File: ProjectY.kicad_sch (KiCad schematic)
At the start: 10 parts, among them J10 NRJ6HF, J2 Conn_ARM_JTAG_SWD_10, J3 9V, J4 NRJ6HF, J5 NRJ6HF, J6 NRJ6HF, J7 SPDIF_OUT, J8 Midi In, J9 MIDI Out, P1 USB_C

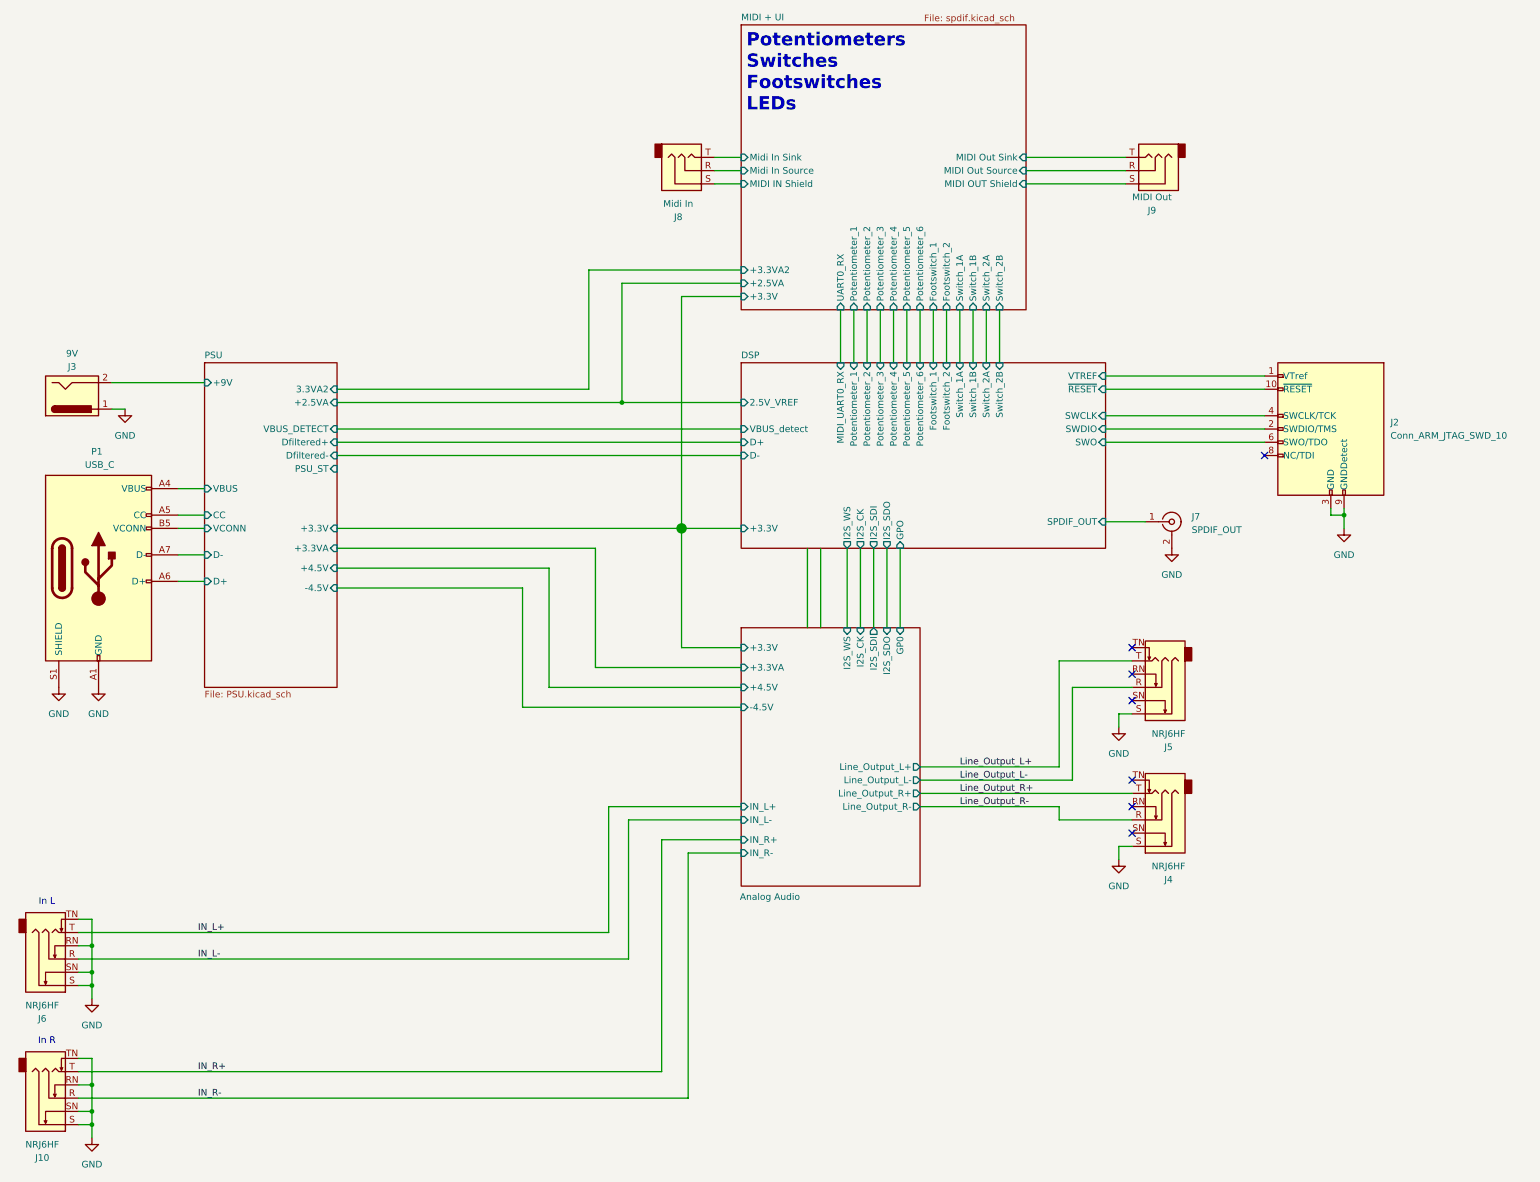
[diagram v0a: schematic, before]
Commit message: started the layout process
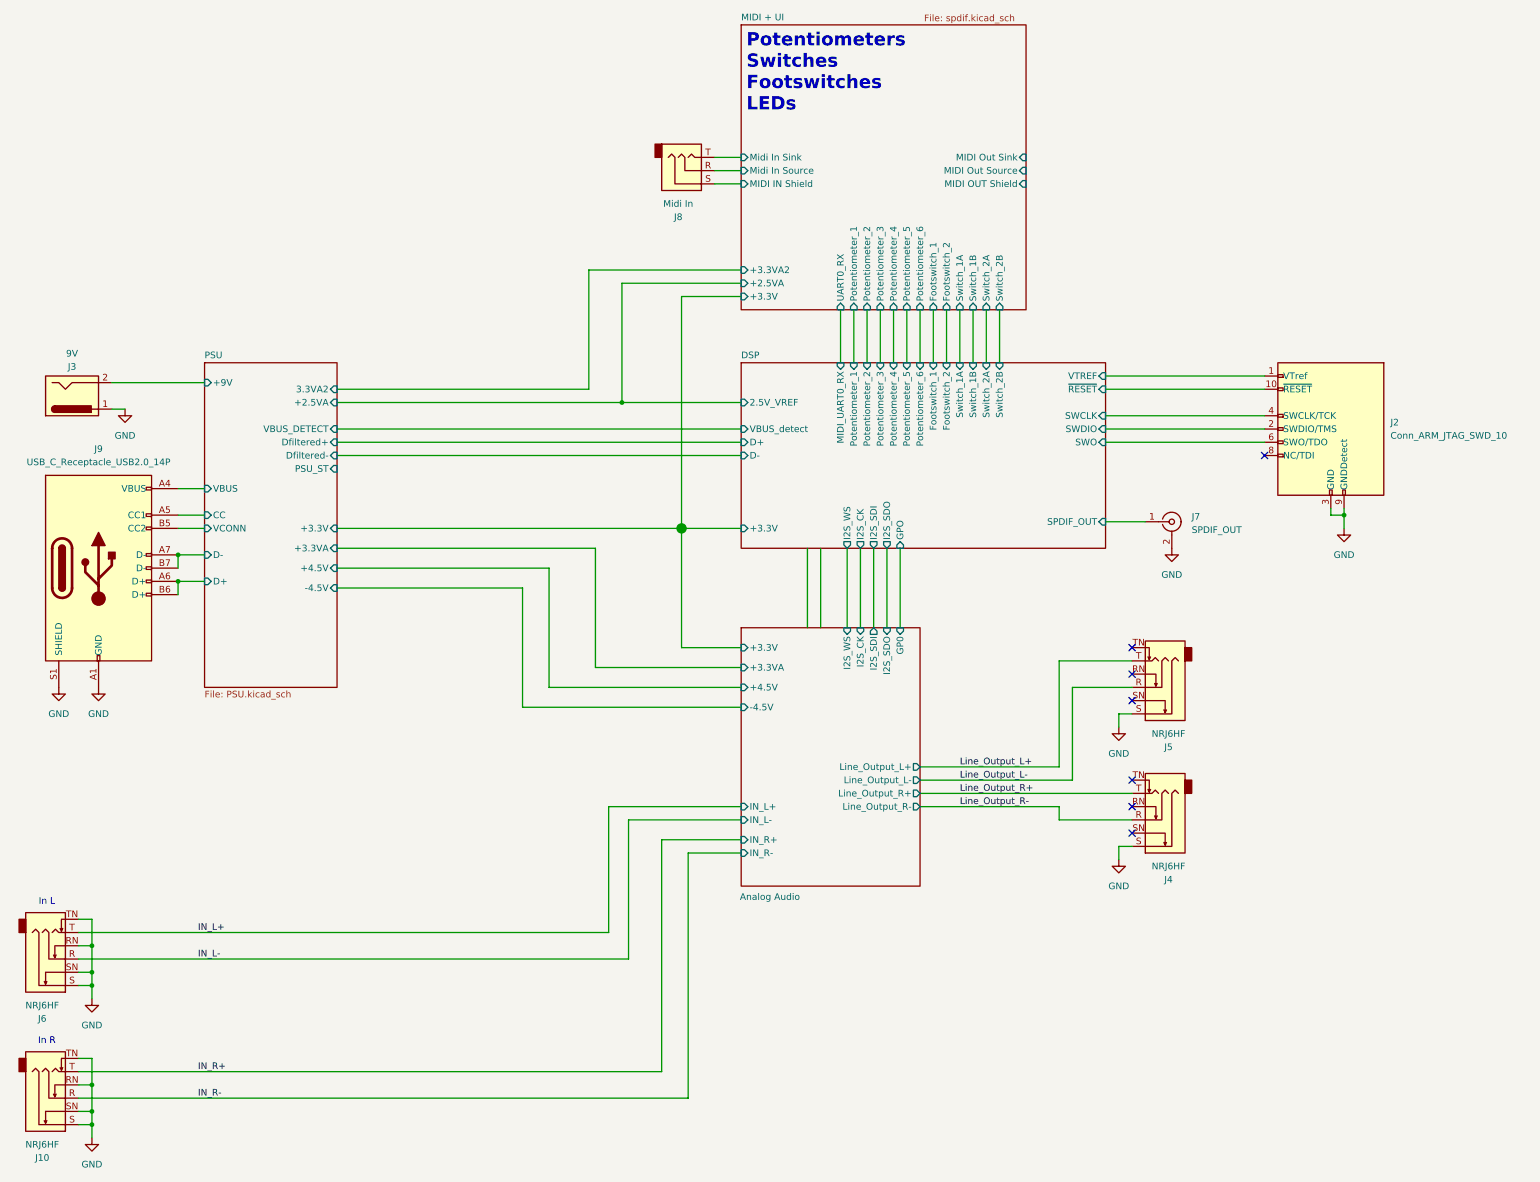
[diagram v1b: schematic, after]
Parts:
- removed J9: MIDI Out, Connector_Audio:Jack_3.5mm_Lumberg_1503_07_Horizontal, symbol Connector_Audio:AudioJack3
- removed P1: USB_C, Connector_USB:USB_C_Receptacle_GCT_USB4110, symbol Connector:USB_C_Plug_USB2.0
- added J9: USB_C_Receptacle_USB2.0_14P, Connector_USB:USB_C_Receptacle_GCT_USB4110, symbol Connector:USB_C_Receptacle_USB2.0_14P
- J2: footprint (none) -> Connector_PinHeader_1.27mm:PinHeader_2x05_P1.27mm_Vertical_SMD
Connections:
- net GND: now also J9.A1 (GND), J9.A12 (GND), J9.B1 (GND), J9.B12 (GND), J9.S1 (SHIELD)
- net PSU/CC: now also J9.A5 (CC1)
- net PSU/D+: now also J9.A6 (D+), J9.B6 (D+)
- net PSU/D-: now also J9.A7 (D-), J9.B7 (D-)
- net PSU/VBUS: now also J9.A4 (VBUS), J9.A9 (VBUS), J9.B4 (VBUS), J9.B9 (VBUS)
- net PSU/VCONN: now also J9.B5 (CC2)
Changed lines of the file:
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@@
+	)
+	(junction
+		(at 100.33 144.78)
+		(diameter 0)
+		(color 0 0 0 0)
 	)
 	(junction
@@
 		(color 255 0 0 1)
 	)
+	(junction
+		(at 100.33 149.86)
+		(diameter 0)
+		(color 0 0 0 0)
+	)
 	(no_connect
 		(at 308.61 125.73)
@@
 	(wire
 		(pts
+			(xy 100.33 147.32) (xy 100.33 144.78)
+		)
+		(stroke
+			(width 0)
+			(type default)
+		)
+	)
+	(wire
+		(pts
 			(xy 283.21 170.18) (xy 271.78 170.18)
 		)
@@
 	(wire
 		(pts
-			(xy 262.89 71.12) (xy 281.94 71.12)
-		)
-		(stroke
-			(width 0)
-			(type default)
-		)
-	)
-	(wire
-		(pts
 			(xy 171.45 147.32) (xy 171.45 170.18)
 		)
@@
 	(wire
 		(pts
+			(xy 100.33 144.78) (xy 105.41 144.78)
+		)
+		(stroke
+			(width 0)
+			(type default)
+		)
+	)
+	(wire
+		(pts
 			(xy 233.68 143.51) (xy 233.68 158.75)
 		)
@@
 	(wire
 		(pts
-			(xy 262.89 73.66) (xy 281.94 73.66)
-		)
-		(stroke
-			(width 0)
-			(type default)
-		)
-	)
-	(wire
-		(pts
 			(xy 182.88 193.04) (xy 208.28 193.04)
 		)
@@
 	(wire
 		(pts
-			(xy 262.89 68.58) (xy 281.94 68.58)
-		)
-		(stroke
-			(width 0)
-			(type default)
-		)
-	)
-	(wire
-		(pts
 			(xy 208.28 95.25) (xy 196.85 95.25)
 		)
@@
 	(wire
 		(pts
-			(xy 100.33 144.78) (xy 105.41 144.78)
-		)
-		(stroke
-			(width 0)
-			(type default)
-		)
-	)
-	(wire
-		(pts
 			(xy 83.82 241.3) (xy 83.82 246.38)
 		)
@@
 		(pts
 			(xy 130.81 147.32) (xy 171.45 147.32)
+		)
+		(stroke
+			(width 0)
+			(type default)
+		)
+	)
+	(wire
+		(pts
+			(xy 100.33 149.86) (xy 100.33 152.4)
 		)
 		(stroke
@@
 	)
 	(symbol
+		(lib_id "Connector:USB_C_Receptacle_USB2.0_14P")
+		(at 85.09 147.32 0)
+		(unit 1)
+		(exclude_from_sim no)
+		(in_bom yes)
+		(on_board yes)
+		(dnp no)
+		(fields_autoplaced yes)
+		(property "Reference" "J9"
+			(at 85.09 124.46 0)
+			(effects
+				(font
+					(size 1.27 1.27)
+				)
+			)
+		)
+		(property "Value" "USB_C_Receptacle_USB2.0_14P"
+			(at 85.09 127 0)
+			(effects
+				(font
+					(size 1.27 1.27)
+				)
+			)
+		)
+		(property "Footprint" "Connector_USB:USB_C_Receptacle_GCT_USB4110"
+			(at 88.9 147.32 0)
+			(effects
+				(font
+					(size 1.27 1.27)
+				)
+				(hide yes)
+			)
+		)
+		(property "Datasheet" "https://www.usb.org/sites/default/files/documents/usb_type-c.zip"
+			(at 88.9 147.32 0)
+			(effects
+				(font
+					(size 1.27 1.27)
+				)
+				(hide yes)
+			)
+		)
+		(property "Description" "USB 2.0-only 14P Type-C Receptacle connector"
+			(at 85.09 147.32 0)
+			(effects
+				(font
+					(size 1.27 1.27)
+				)
+				(hide yes)
+			)
+		)
+		(pin "B5"
+		)
+		(pin "A5"
+		)
+		(pin "A1"
+		)
+		(pin "A9"
+		)
+		(pin "A4"
+		)
+		(pin "A12"
+		)
+		(pin "B1"
+		)
+		(pin "B12"
+		)
+		(pin "B4"
+		)
+		(pin "S1"
+		)
+		(pin "B9"
+		)
+		(pin "A6"
+		)
+		(pin "A7"
+		)
+		(pin "B7"
+		)
+		(pin "B6"
+		)
+		(instances
+			(project ""
+				(path "/6b669608-d244-47fa-b233-c11102b937f7"
+					(reference "J9")
+					(unit 1)
+				)
+			)
+		)
+	)
+	(symbol
 		(lib_id "power:GND")
 		(at 83.82 229.87 0)
@@
 				(path "/6b669608-d244-47fa-b233-c11102b937f7"
 					(reference "J3")
-					(unit 1)
-				)
-			)
-		)
-	)
-	(symbol
-		(lib_id "Connector_Audio:AudioJack3")
-		(at 287.02 71.12 180)
-		(unit 1)
-		(exclude_from_sim no)
-		(in_bom yes)
-		(on_board yes)
-		(dnp no)
-		(property "Reference" "J9"
-			(at 287.02 78.74 0)
-			(effects
-				(font
-					(size 1.27 1.27)
-				)
-			)
-		)
-		(property "Value" "MIDI Out"
-			(at 287.02 76.2 0)
-			(effects
-				(font
-					(size 1.27 1.27)
-				)
-			)
-		)
-		(property "Footprint" "Connector_Audio:Jack_3.5mm_Lumberg_1503_07_Horizontal"
-			(at 287.02 71.12 0)
-			(effects
-				(font
-					(size 1.27 1.27)
-				)
-				(hide yes)
-			)
-		)
-		(property "Datasheet" "~"
-			(at 287.02 71.12 0)
-			(effects
-				(font
-					(size 1.27 1.27)
-				)
-				(hide yes)
-			)
-		)
-		(property "Description" "Audio Jack, 3 Poles (Stereo / TRS)"
-			(at 287.02 71.12 0)
-			(effects
-				(font
-					(size 1.27 1.27)
-				)
-				(hide yes)
-			)
-		)
-		(pin "R"
-		)
-		(pin "S"
-		)
-		(pin "T"
-		)
-		(instances
-			(project "ProjectY"
-				(path "/6b669608-d244-47fa-b233-c11102b937f7"
-					(reference "J9")
-					(unit 1)
-				)
-			)
-		)
-	)
-	(symbol
-		(lib_id "Connector:USB_C_Plug_USB2.0")
-		(at 85.09 147.32 0)
-		(unit 1)
-		(exclude_from_sim no)
-		(in_bom yes)
-		(on_board yes)
-		(dnp no)
-		(property "Reference" "P1"
-			(at 85.852 124.968 0)
-			(effects
-				(font
-					(size 1.27 1.27)
-				)
-				(justify right)
-			)
-		)
-		(property "Value" "USB_C"
-			(at 88.138 127.508 0)
-			(effects
-				(font
-					(size 1.27 1.27)
-				)
-				(justify right)
-			)
-		)
-		(property "Footprint" "Connector_USB:USB_C_Receptacle_GCT_USB4110"
-			(at 88.9 147.32 0)
-			(effects
-				(font
-					(size 1.27 1.27)
-				)
-				(hide yes)
-			)
-		)
-		(property "Datasheet" "https://www.usb.org/sites/default/files/documents/usb_type-c.zip"
-			(at 88.9 147.32 0)
-			(effects
-				(font
-					(size 1.27 1.27)
-				)
-				(hide yes)
-			)
-		)
-		(property "Description" "USB 2.0-only Type-C Plug connector"
-			(at 85.09 147.32 0)
-			(effects
-				(font
-					(size 1.27 1.27)
-				)
-				(hide yes)
-			)
-		)
-		(pin "A5"
-		)
-		(pin "A6"
-		)
-		(pin "B4"
-		)
-		(pin "A9"
-		)
-		(pin "B1"
-		)
-		(pin "S1"
-		)
-		(pin "A7"
-		)
-		(pin "A12"
-		)
-		(pin "B12"
-		)
-		(pin "A1"
-		)
-		(pin "B9"
-		)
-		(pin "B5"
-		)
-		(pin "A4"
-		)
-		(instances
-			(project "ProjectY"
-				(path "/6b669608-d244-47fa-b233-c11102b937f7"
-					(reference "P1")
 					(unit 1)
 				)
@@
 			)
 		)
-		(property "Footprint" ""
+		(property "Footprint" "Connector_PinHeader_1.27mm:PinHeader_2x05_P1.27mm_Vertical_SMD"
 			(at 321.31 120.65 0)
 			(effects
@@
 	(symbol
 		(lib_id "power:GND")
-		(at 77.47 170.18 0)
+		(at 85.09 170.18 0)
 		(unit 1)
 		(exclude_from_sim no)
@@
 		(dnp no)
 		(fields_autoplaced yes)
-		(property "Reference" "#PWR039"
-			(at 77.47 176.53 0)
+		(property "Reference" "#PWR038"
+			(at 85.09 176.53 0)
 			(effects
 				(font
@@
 		)
 		(property "Value" "GND"
-			(at 77.47 175.26 0)
+			(at 85.09 175.26 0)
 			(effects
 				(font
@@
 		)
 		(property "Footprint" ""
-			(at 77.47 170.18 0)
+			(at 85.09 170.18 0)
 			(effects
 				(font
@@
 		)
 		(property "Datasheet" ""
-			(at 77.47 170.18 0)
+			(at 85.09 170.18 0)
 			(effects
 				(font
@@
 		)
 		(property "Description" "Power symbol creates a global label with name \"GND\" , ground"
-			(at 77.47 170.18 0)
+			(at 85.09 170.18 0)
 			(effects
 				(font
@@
 			(project "ProjectY"
 				(path "/6b669608-d244-47fa-b233-c11102b937f7"
-					(reference "#PWR039")
+					(reference "#PWR038")
 					(unit 1)
 				)
@@
 	(symbol
 		(lib_id "power:GND")
-		(at 85.09 170.18 0)
+		(at 77.47 170.18 0)
 		(unit 1)
 		(exclude_from_sim no)
@@
 		(dnp no)
 		(fields_autoplaced yes)
-		(property "Reference" "#PWR038"
-			(at 85.09 176.53 0)
+		(property "Reference" "#PWR039"
+			(at 77.47 176.53 0)
 			(effects
 				(font
@@
 		)
 		(property "Value" "GND"
-			(at 85.09 175.26 0)
+			(at 77.47 175.26 0)
 			(effects
 				(font
@@
 		)
 		(property "Footprint" ""
-			(at 85.09 170.18 0)
+			(at 77.47 170.18 0)
 			(effects
 				(font
@@
 		)
 		(property "Datasheet" ""
-			(at 85.09 170.18 0)
+			(at 77.47 170.18 0)
 			(effects
 				(font
@@
 		)
 		(property "Description" "Power symbol creates a global label with name \"GND\" , ground"
-			(at 85.09 170.18 0)
+			(at 77.47 170.18 0)
 			(effects
 				(font
@@
 			(project "ProjectY"
 				(path "/6b669608-d244-47fa-b233-c11102b937f7"
-					(reference "#PWR038")
+					(reference "#PWR039")
 					(unit 1)
 				)

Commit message: lot of changes
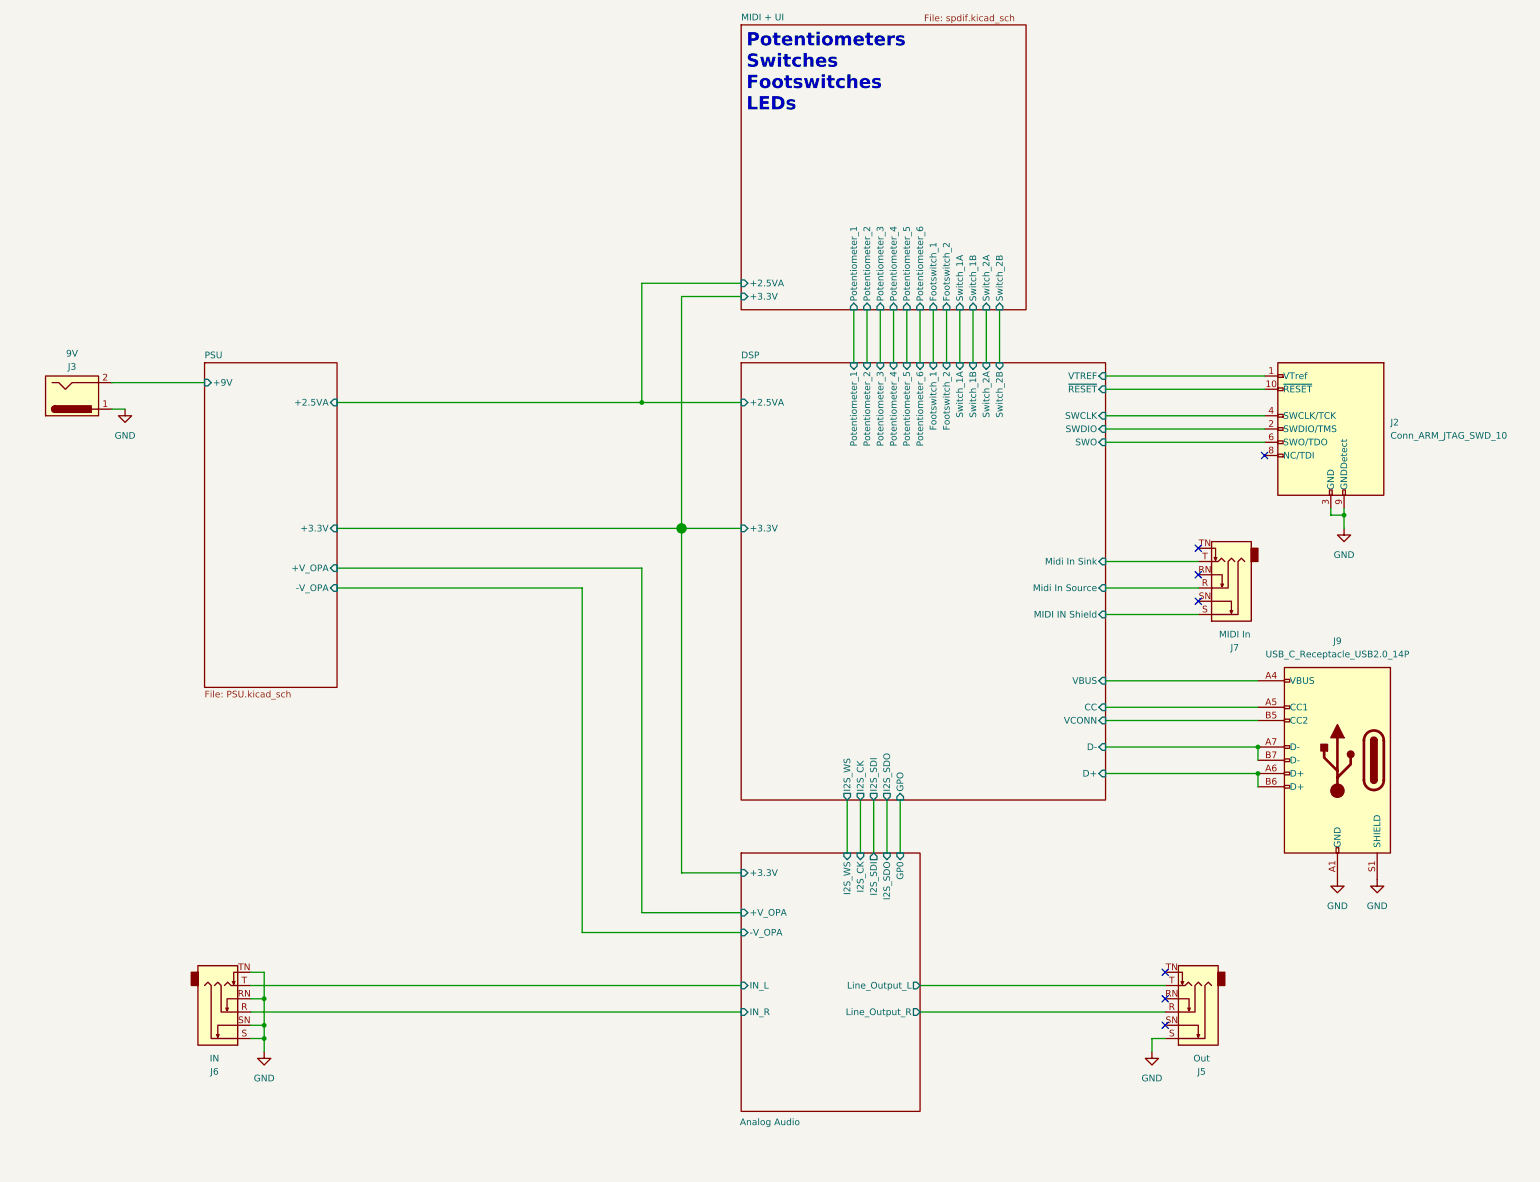
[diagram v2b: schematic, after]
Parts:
- removed J10, J4: NRJ6HF, Connector_Audio:Jack_6.35mm_Neutrik_NRJ6HF_Horizontal, symbol Connector_Audio:NRJ6HF
- removed J7: SPDIF_OUT, symbol Connector:Conn_Coaxial
- removed J8: Midi In, Connector_Audio:Jack_3.5mm_Lumberg_1503_07_Horizontal, symbol Connector_Audio:AudioJack3
- added J7: MIDI In, User:Jack_6.35mm_Neutrik_NRJ6HF_Horizontal, symbol Connector_Audio:NRJ6HF
- J3: footprint Connector_BarrelJack:BarrelJack_GCT_DCJ200-10-A_Horizontal -> User:BarrelJack_GCT_DCJ200-10-A_Horizontal
- J5: value NRJ6HF -> Out; footprint Connector_Audio:Jack_6.35mm_Neutrik_NRJ6HF_Horizontal -> User:Jack_6.35mm_Neutrik_NRJ6HF_Horizontal; PN (none) -> NRJ6HF
- J6: value NRJ6HF -> IN; footprint Connector_Audio:Jack_6.35mm_Neutrik_NRJ6HF_Horizontal -> User:Jack_6.35mm_Neutrik_NRJ6HF_Horizontal; PN (none) -> NRJ6HF
- J9: footprint Connector_USB:USB_C_Receptacle_GCT_USB4110 -> User:USB_C_Receptacle_GCT_USB4110
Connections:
- net PSU/D+ is gone; now on net DSP/D+: J9.A6 (D+), J9.B6 (D+)
- net PSU/D- is gone; now on net DSP/D-: J9.A7 (D-), J9.B7 (D-)
- net IN_L+ renamed Analog Audio/IN_L
- net IN_L- renamed Analog Audio/IN_R
- net Line_Output_L+ renamed Analog Audio/Line_Output_L
- net Line_Output_L- renamed Analog Audio/Line_Output_R
- net PSU/CC renamed DSP/CC
- net PSU/VBUS renamed DSP/VBUS
- net PSU/VCONN renamed DSP/VCONN
- new net DSP/MIDI IN Shield: J7.S
- new net DSP/Midi In Sink: J7.T
- new net DSP/Midi In Source: J7.R
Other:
- sheet Analog Audio ports: added +V_OPA, -V_OPA, IN_L, IN_R, Line_Output_L, Line_Output_R; removed +3.3VA, +4.5V, -4.5V, IN_L+, IN_L-, IN_R+, IN_R-, Line_Output_L+, Line_Output_L-, Line_Output_R+, Line_Output_R-
- sheet DSP ports: added +2.5VA, CC, MIDI IN Shield, Midi In Sink, Midi In Source, VBUS, VCONN; removed 2.5V_VREF, MIDI_UART0_RX, SPDIF_OUT, VBUS_detect
- sheet MIDI + UI ports: added none; removed +3.3VA2, MIDI IN Shield, MIDI OUT Shield, MIDI Out Sink, MIDI Out Source, Midi In Sink, Midi In Source, UART0_RX
- sheet PSU ports: added +V_OPA, -V_OPA; removed +3.3VA, +4.5V, -4.5V, 3.3VA2, CC, D+, D-, Dfiltered+, Dfiltered-, PSU_ST, VBUS, VBUS_DETECT, VCONN
- note removed: "In L"
- note removed: "In R"
- moved on the sheet: J5, J6, J9
